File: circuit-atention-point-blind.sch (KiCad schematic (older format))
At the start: 27 parts

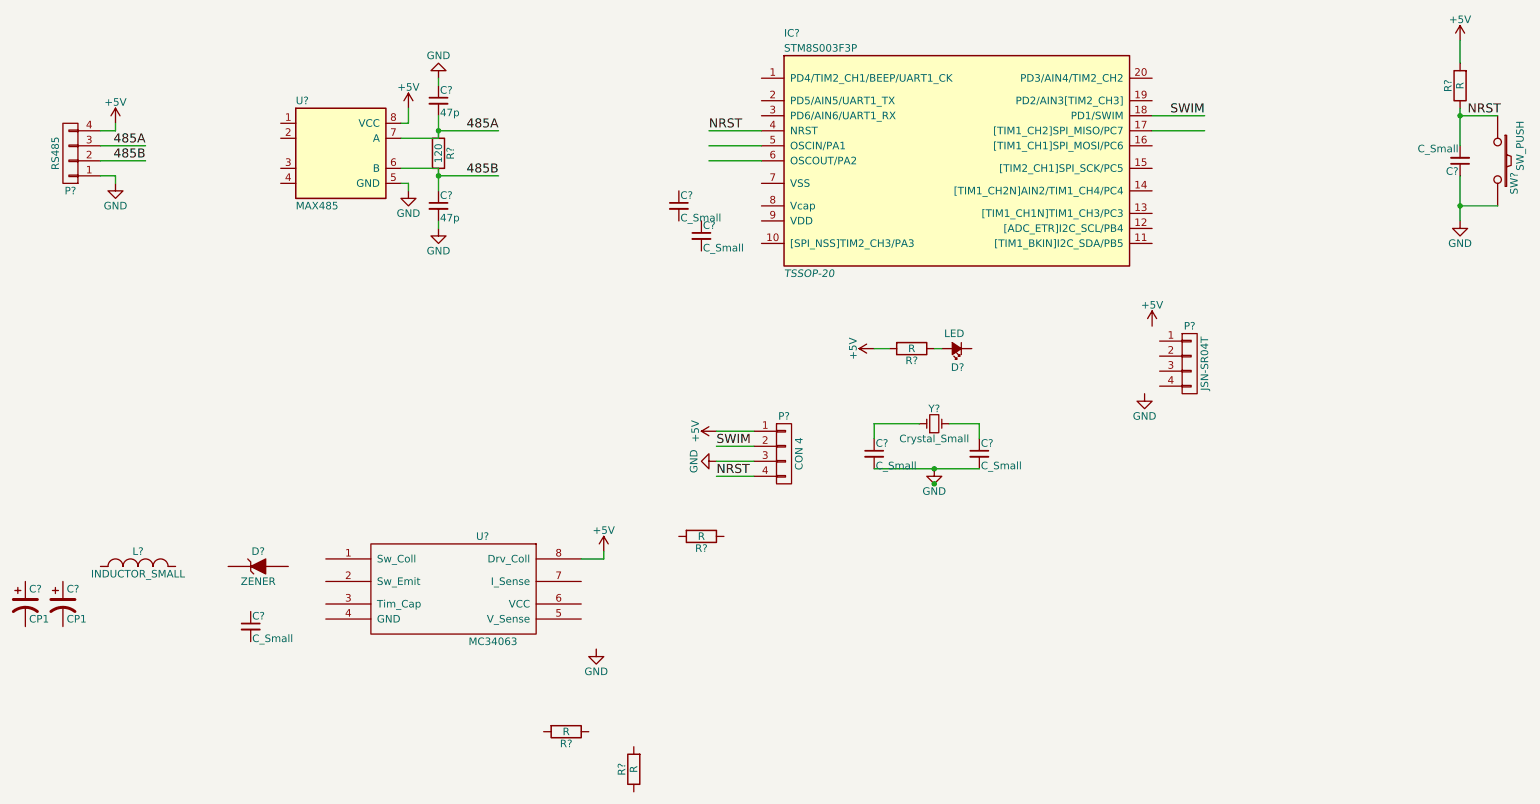
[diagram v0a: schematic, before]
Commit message: modify sch
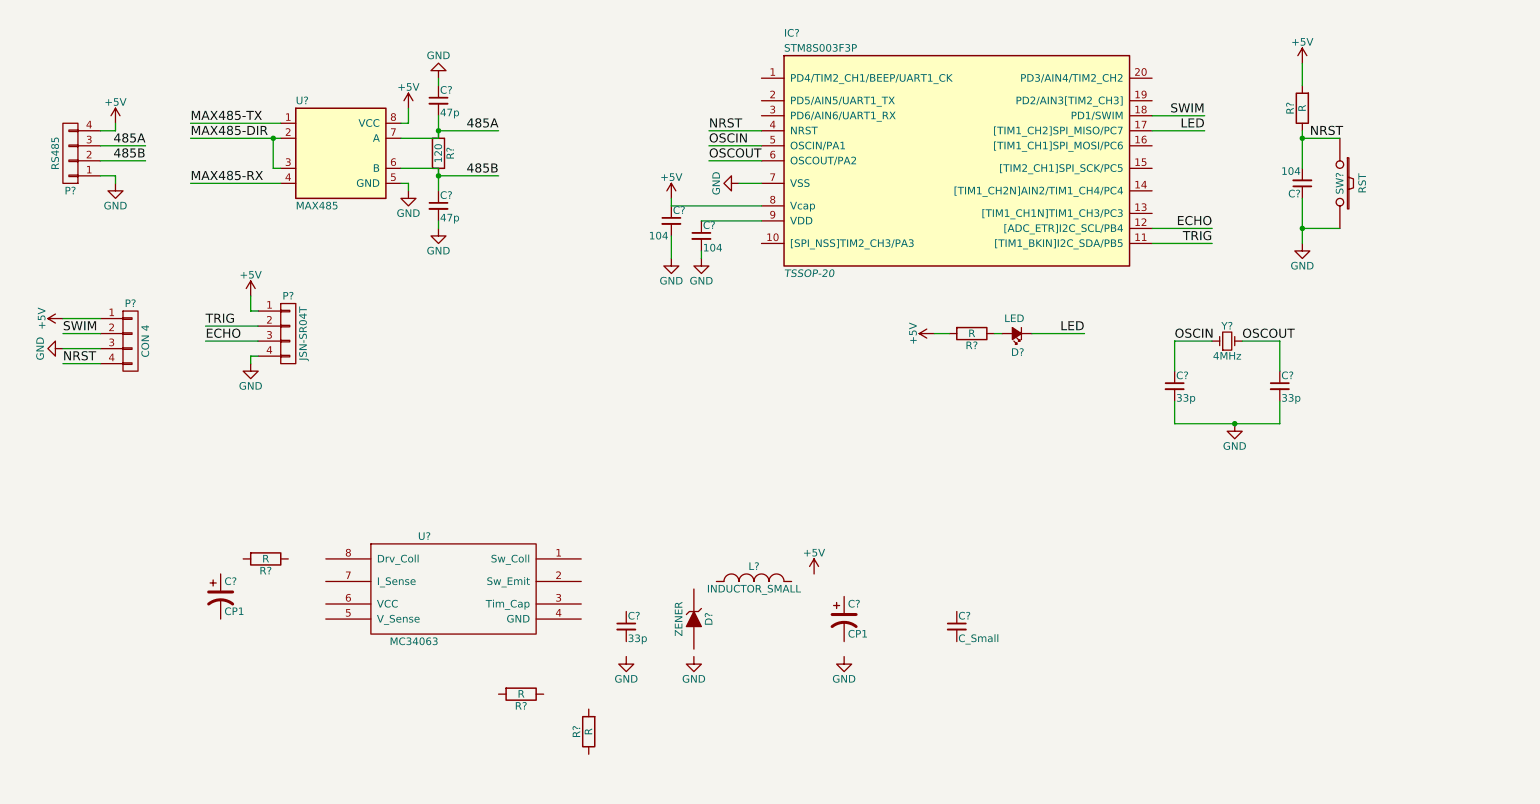
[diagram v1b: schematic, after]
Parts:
- added C?: 33p, symbol C_Small
- C? (x3): value C_Small -> 104
- C? (x2): value C_Small -> 33p
- SW?: value SW_PUSH -> RST
- Y?: value Crystal_Small -> 4MHz
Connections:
- net labels added: ECHO, LED, MAX485-DIR, MAX485-RX, MAX485-TX, OSCIN, OSCOUT, TRIG
- wire segments 41 -> 61
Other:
- moved on the sheet: C?, D?, L?, P?, R?, SW?, Y?

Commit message: initial PCB
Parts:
- removed C? (x2): 33p, symbol C_Small
- removed C?: 104, symbol C_Small
- removed C?: C_Small, symbol C_Small
- removed R?: R, symbol R
- removed SW?: RST, symbol SW_PUSH
- removed Y?: 4MHz, symbol Crystal_Small
- added C8: 104, Capacitors_SMD:C_0805_HandSoldering, symbol C_Small
- added D2: LED, LEDs:LED_0805, symbol Led_Small
- added D4: SS14, Diodes_SMD:DO-214BA, symbol D_Small
- added R2: R, Resistors_SMD:R_0805_HandSoldering, symbol R
- added R3: 10k, Resistors_SMD:R_0805_HandSoldering, symbol R
- 0.33, 1k-1%1, 3k-1%1, R1: renamed from R?; footprint (none) -> Resistors_SMD:R_0805_HandSoldering
- C1: renamed from C?; value CP1 -> 470u; footprint (none) -> Capacitors_SMD:c_elec_10x10
- C2, C3, C6: renamed from C?; footprint (none) -> Capacitors_SMD:C_0805_HandSoldering
- C4, C5: renamed from C?; value 104 -> 1u; footprint (none) -> Capacitors_SMD:C_0805_HandSoldering
- C7: renamed from C?; value CP1 -> 470u; footprint (none) -> Capacitors_SMD:c_elec_6.3x5.7
- D1: renamed from D?; value ZENER -> 1N5819; footprint (none) -> Diodes_SMD:MELF_Standard
- D3: renamed from D?; footprint (none) -> LEDs:LED_0805
- IC1: renamed from IC?; footprint TSSOP-20 -> Housings_SSOP:TSSOP-20_4.4x6.5mm_Pitch0.65mm; symbol STM8S003F3P -> STM8S003F3P-RESCUE-circuit-atention-point-blind
- L1: renamed from L?; value INDUCTOR_SMALL -> 100uH; footprint (none) -> Inductors_NEOSID:Neosid_Inductor_SM1206
- P1: renamed from P?; footprint (none) -> Connectors_Molex:Molex_KK_6410-04
- P2, P3: renamed from P?; footprint (none) -> Pin_Headers:Pin_Header_Angled_1x04
- R4: renamed from R?; value R -> 1K; footprint (none) -> Resistors_SMD:R_0805_HandSoldering
- U1: renamed from U?; footprint (none) -> Housings_SOIC:SOIC-8_3.9x4.9mm_Pitch1.27mm; symbol MAX471 -> MAX471-RESCUE-circuit-atention-point-blind
- U2: renamed from U?; footprint (none) -> Housings_SOIC:SOIC-8_3.9x4.9mm_Pitch1.27mm; symbol MC34063 -> MC34063-RESCUE-circuit-atention-point-blind
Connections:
- net NRST is gone; now on net +5V: IC1.4 (NRST), P2.4 (P4)
- net +5V: now also 3k-1%1.2, C7.1, IC1.9 (VDD), L1.2, D2.2 (A), R3.1; no longer IC1.8 (Vcap), P1.4 (P4)
- net ECHO: now also IC1.11 ([TIM1_BKIN]I2C_SDA/PB5); no longer IC1.12 ([ADC_ETR]I2C_SCL/PB4)
- net GND: now also 1k-1%1.1, C1.2, C6.2, C7.2, D1.2 (A), U2.4 (GND), C8.2, R2.1
- net MAX485-DIR: now also IC1.14 ([TIM1_CH2N]AIN2/TIM1_CH4/PC4)
- net MAX485-RX: now also IC1.3 (PD6/AIN6/UART1_RX), U1.1; no longer U1.4
- net MAX485-TX: now also IC1.2 (PD5/AIN5/UART1_TX), U1.4; no longer U1.1
- net TRIG: now also IC1.1 (PD4/TIM2_CH1/BEEP/UART1_CK); no longer IC1.11 ([TIM1_BKIN]I2C_SDA/PB5)
- net at C5.1: now also IC1.8 (Vcap); no longer IC1.9 (VDD)
- net at U2.1 (Sw_Coll): now also 0.33.1, U2.7 (I_Sense), U2.8 (Drv_Coll)
- net at U2.2 (Sw_Emit): now also D1.1 (K), L1.1
- net at U2.3 (Tim_Cap): now also C6.1
- net at U2.5 (V_Sense): now also 1k-1%1.2, 3k-1%1.1
- net +24V: now reaches U2.6 (VCC)
- net +24V: now also C1.1, P1.4 (P4), D4.2 (A)
- net at 0.33.2: now also D4.1 (K)
- net LED: no longer names the net of D3.1 (K), IC1.17 ([TIM1_CH2]SPI_MISO/PC7)
- net OSCIN: no longer names the net of IC1.5 (OSCIN/PA1)
- net OSCOUT: no longer names the net of IC1.6 (OSCOUT/PA2)
- new net: D2.1 (K), R2.2
- new net: C8.1, R3.2
- no-connect marks 0 -> 9
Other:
- moved on the sheet: 0.33, 1k-1%1, 3k-1%1, C1, C4, C5, C6, C7, D1, D3, L1, R4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
